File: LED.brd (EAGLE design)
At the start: 31.8 x 21.5 mm, 8 parts, among them J1 CONECTOR_MACHO, J2 CONECTOR_FEMEA, Q1 BC817, U1 74HC132

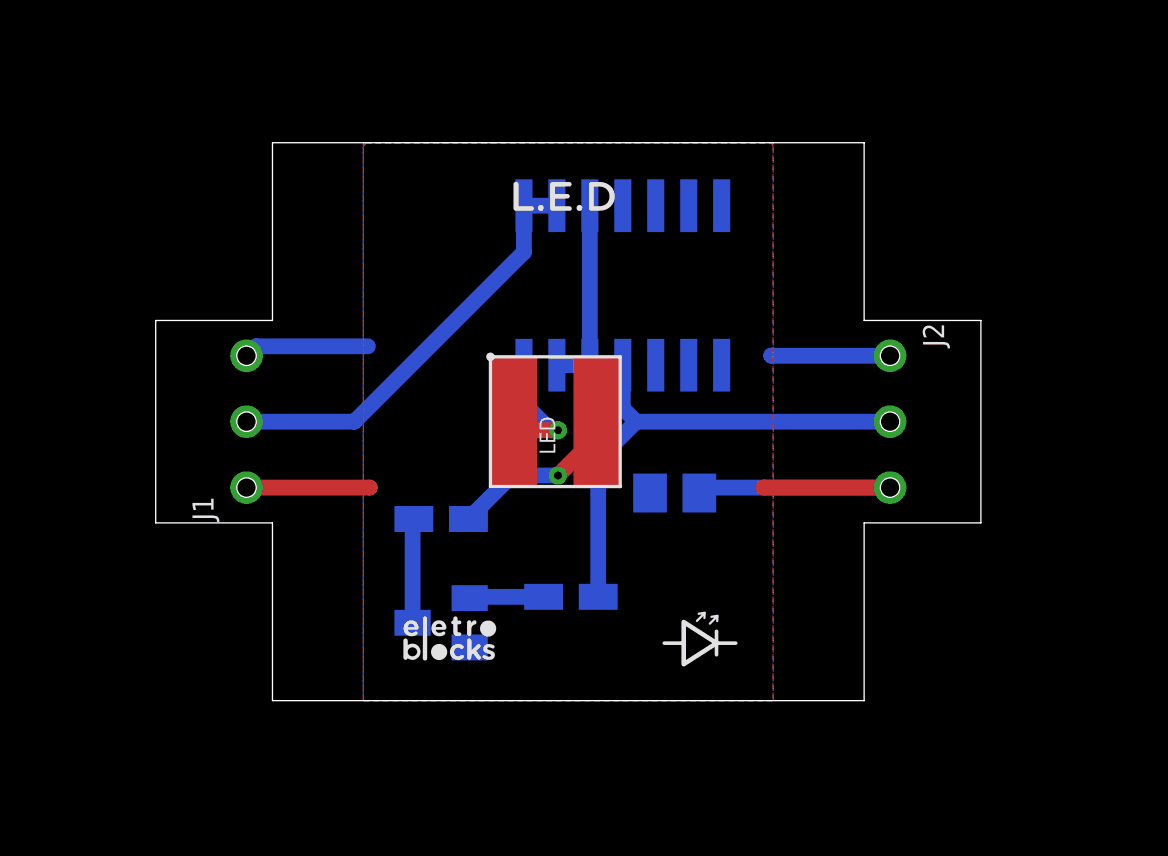
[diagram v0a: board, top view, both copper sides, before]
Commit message: V1.0.3
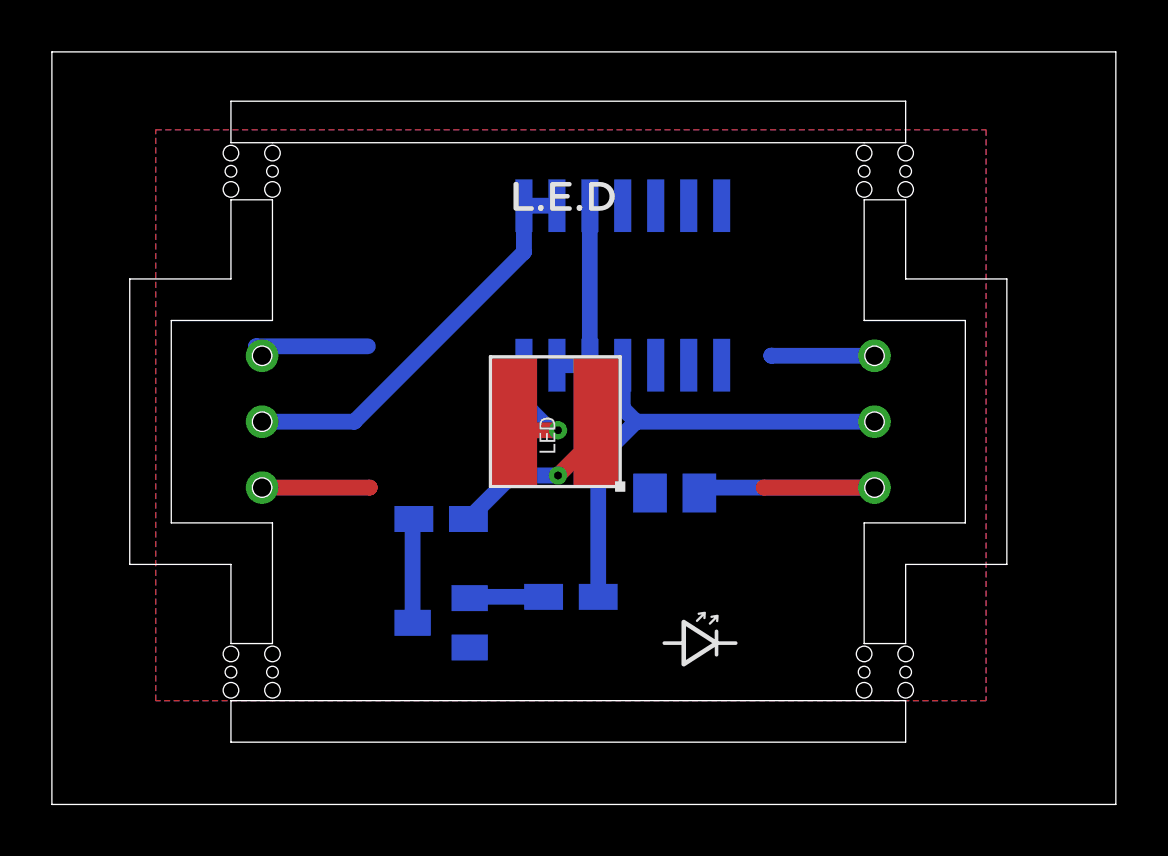
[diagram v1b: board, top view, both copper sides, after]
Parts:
- added U$2, U$3, U$4, U$5: (no value), Eletroblocks Lib:STAMP_DUPLO
- J1: device Eletroblocks Lib:3CONECTOR -> Eletroblocks Lib:MALE
- J2: device Eletroblocks Lib:3CONECTOR -> Eletroblocks Lib:FEMALE
- moved J2 0.60 mm to (19.7, 10.8)
- moved J1 0.60 mm to (-3.90, 10.8)
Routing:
- net VCC: track 22.1 -> 20.3 mm
- net GND: track 9.42 -> 8.73 mm
- net SIGNAL_OUT: track 19.5 -> 18.9 mm
- net SIGNAL_IN: track 16.5 -> 15.9 mm
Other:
- board size 31.8 x 21.5 mm -> 41 x 29 mm
- board text added: "V1.0.2"
- board text removed: "V1.0.1"
